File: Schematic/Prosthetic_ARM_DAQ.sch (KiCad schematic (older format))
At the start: 12 parts, among them J1 USB4085-GF-A_REVA, J2 Conn_01x05, U1 STM32F411CEUx

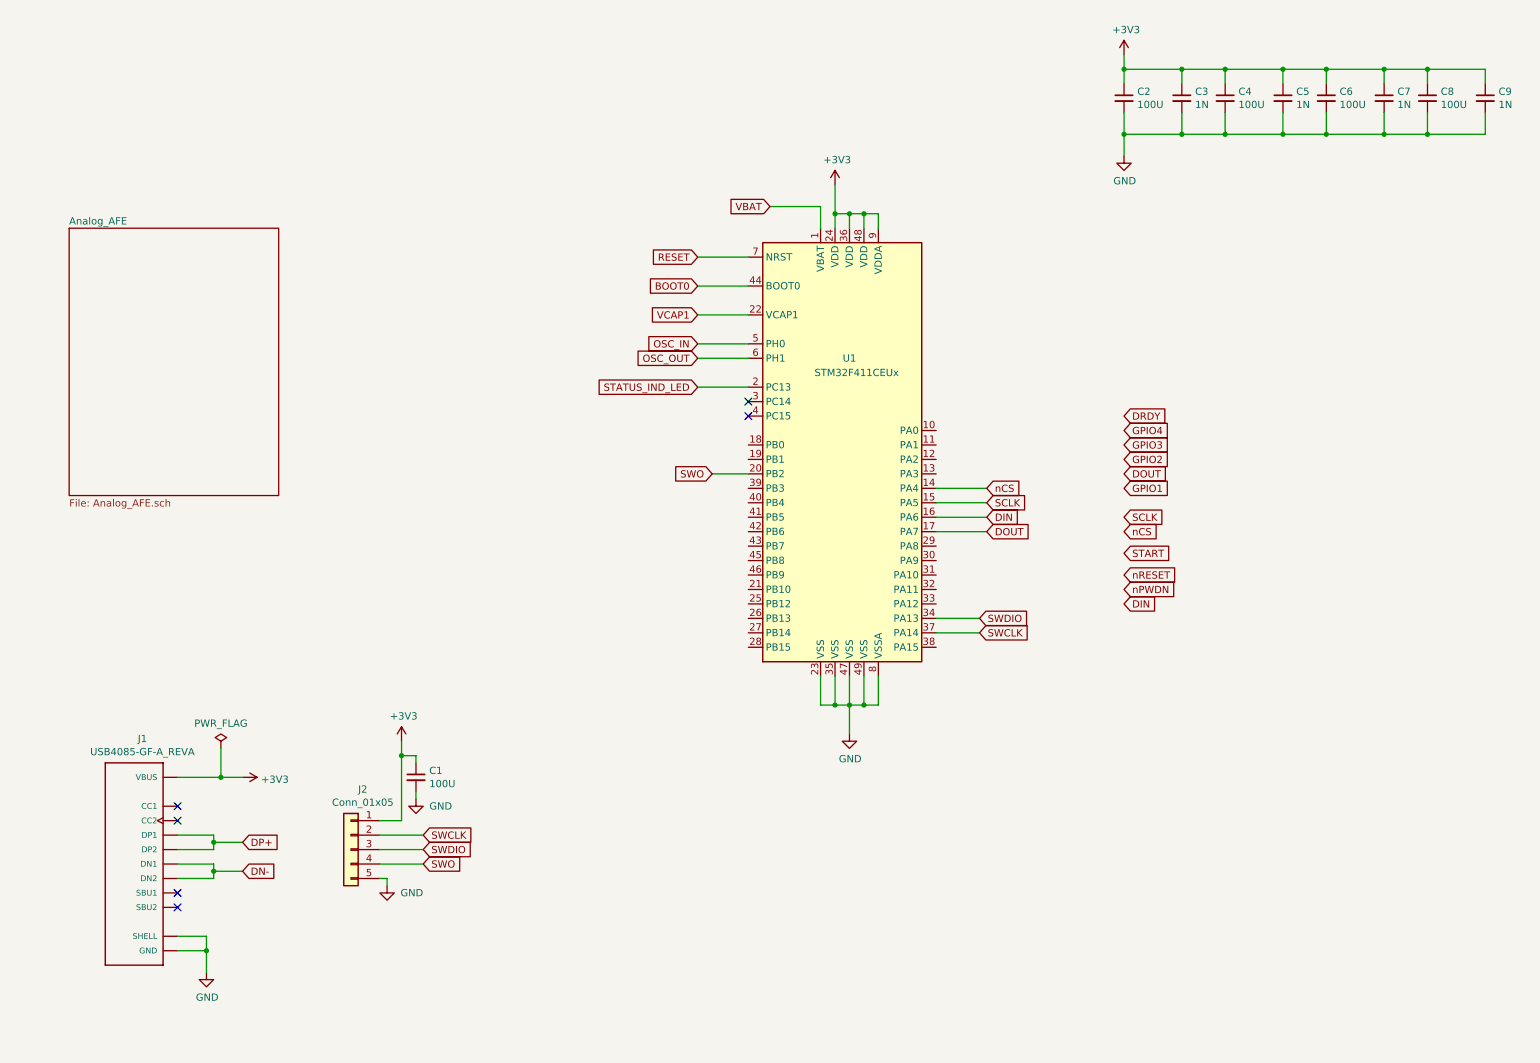
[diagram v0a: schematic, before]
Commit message: Add files via upload
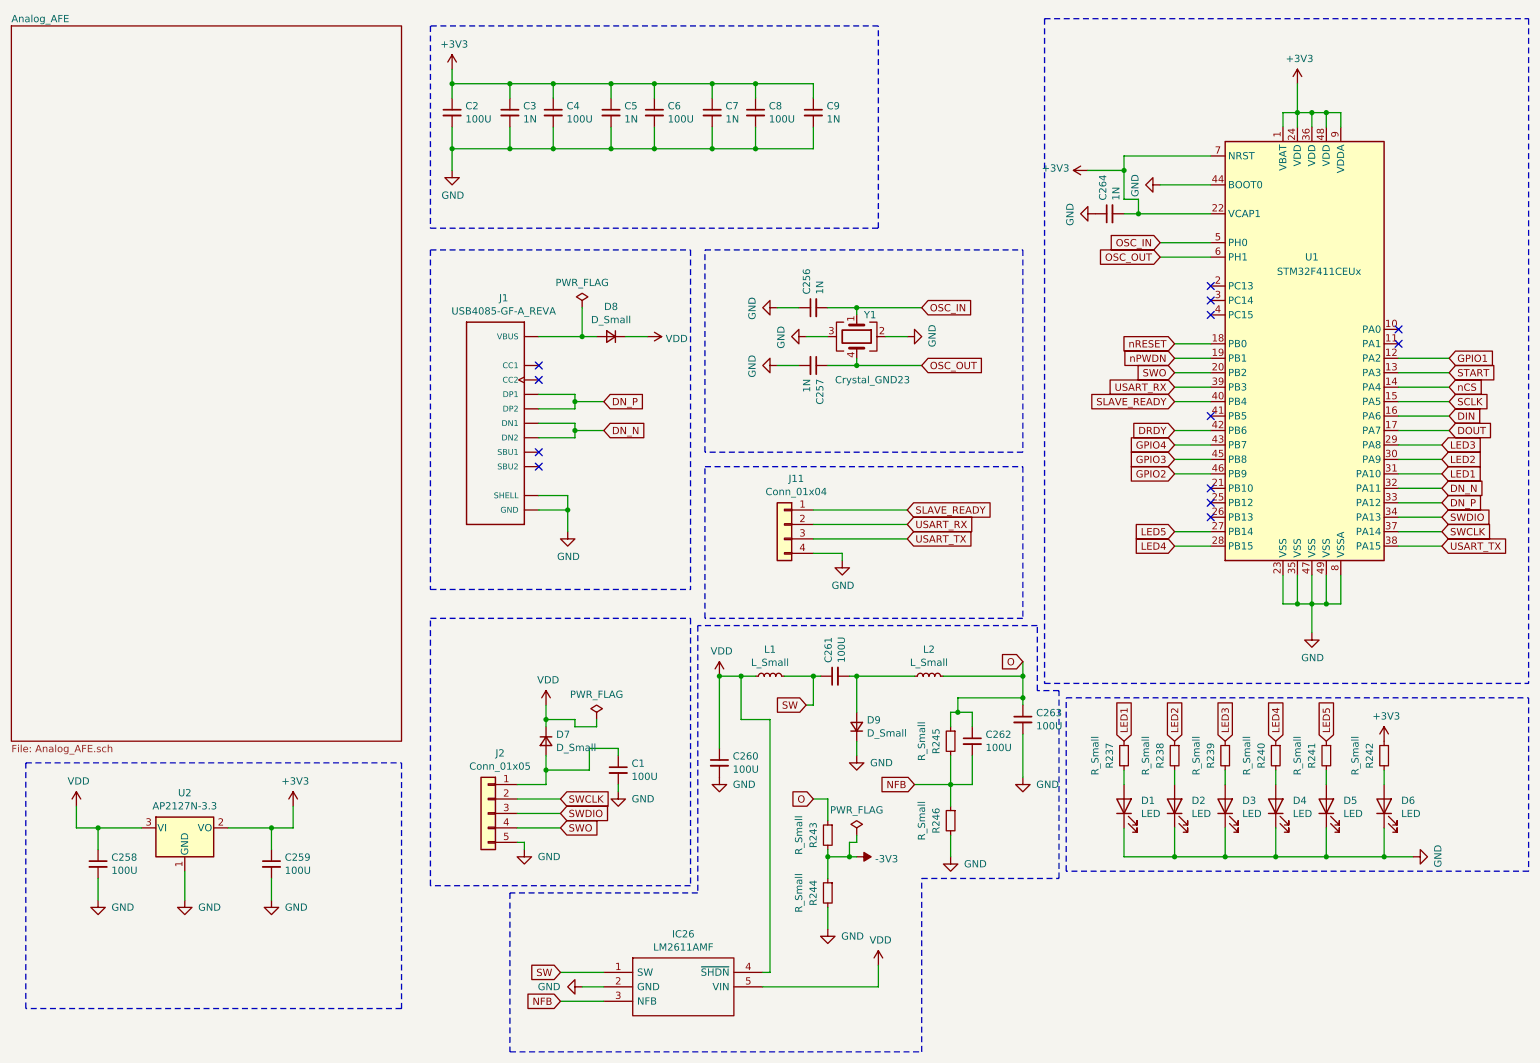
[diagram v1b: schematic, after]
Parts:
- added C256, C257, C264: 1N, Capacitor_SMD:C_0402_1005Metric, symbol Device:C_Small
- added C258, C259, C260, C261, C262, C263: 100U, Capacitor_SMD:C_0402_1005Metric, symbol Device:C_Small
- added D1, D2, D3, D4, D5, D6: LED, LED_SMD:LED_0805_2012Metric_Pad1.15x1.40mm_HandSolder, symbol Device:LED
- added D7, D8, D9: D_Small, Diode_SMD:D_0603_1608Metric_Pad1.05x0.95mm_HandSolder, symbol Device:D_Small
- added IC26: LM2611AMF, ASSETS:SOT95P280X145-5N, symbol Regular_Use:LM2611AMF
- added J11: Conn_01x04, Connector_JST:JST_PH_B4B-PH-SM4-TB_1x04-1MP_P2.00mm_Vertical, symbol Connector_Generic:Conn_01x04
- added L1, L2: L_Small, Inductor_SMD:L_0603_1608Metric_Pad1.05x0.95mm_HandSolder, symbol Device:L_Small
- added R237, R238, R239, R240, R241, R242, R243, R244, R245, R246: R_Small, Resistor_SMD:R_0402_1005Metric, symbol Device:R_Small
- added U2: AP2127N-3.3, Package_TO_SOT_SMD:SOT-23, symbol Regulator_Linear:AP2127N-3.3
- added Y1: Crystal_GND23, Crystal:Crystal_SMD_TXC_7M-4Pin_3.2x2.5mm, symbol Device:Crystal_GND23
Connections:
- net BOOT0 is gone; now on net GND: U1.44 (BOOT0)
- net DN- is gone; now on net DN_N: J1.A7 (DN1), J1.B7 (DN2)
- net DP+ is gone; now on net DN_P: J1.A6 (DP1), J1.B6 (DP2)
- net RESET is gone; now on net +3V3: U1.7 (NRST)
- net VBAT is gone; now on net +3V3: U1.1 (VBAT)
- net VCAP1 is gone; now on net +3V3: U1.22 (VCAP1)
- net +3V3: now also C259.1, C264.2, R242.1, U2.2 (VO); no longer C1.1, J1.A4 (VBUS), J1.A9 (VBUS), J1.B4 (VBUS), J1.B9 (VBUS), J2.1 (Pin_1)
- net DRDY: now also U1.42 (PB6)
- net GND: now also C256.1, C257.2, C258.2, C259.2, C260.2, C263.2, C264.1, D1.1 (K), D2.1 (K), D3.1 (K), D4.1 (K), D5.1 (K), D6.1 (K), D9.1 (K), IC26.2 (GND), J11.4 (Pin_4), R244.2, R246.2, U2.1 (GND), Y1.2, Y1.3
- net GPIO1: now also U1.12 (PA2)
- net GPIO2: now also U1.46 (PB9)
- net GPIO3: now also U1.45 (PB8)
- net GPIO4: now also U1.43 (PB7)
- net OSC_IN: now also C256.2, Y1.1
- net OSC_OUT: now also C257.1, Y1.4
- net START: now also U1.13 (PA3)
- net nPWDN: now also U1.19 (PB1)
- net nRESET: now also U1.18 (PB0)
- net LED5: now reaches U1.27 (PB14)
- net LED5: now also R241.1
- net LED4: now reaches U1.28 (PB15)
- net LED4: now also R240.1
- net LED3: now reaches U1.29 (PA8)
- net LED3: now also R239.1
- net LED2: now reaches U1.30 (PA9)
- net LED2: now also R238.1
- net LED1: now reaches U1.31 (PA10)
- net LED1: now also R237.1
- net DN_N: now reaches U1.32 (PA11)
- net DN_P: now reaches U1.33 (PA12)
- net USART_TX: now reaches U1.38 (PA15)
- net USART_TX: now also J11.3 (Pin_3)
- net USART_RX: now reaches U1.39 (PB3)
- net USART_RX: now also J11.2 (Pin_2)
- net SLAVE_READY: now reaches U1.40 (PB4)
- net SLAVE_READY: now also J11.1 (Pin_1)
- net STATUS_IND_LED: no longer names the net of U1.2 (PC13)
- new net: C1.1, D7.2 (A), J2.1 (Pin_1)
- new net: D8.2 (A), J1.A4 (VBUS), J1.A9 (VBUS), J1.B4 (VBUS), J1.B9 (VBUS)
- new net: D1.2 (A), R237.2
- new net: D2.2 (A), R238.2
- new net: D3.2 (A), R239.2
- new net: D4.2 (A), R240.2
- new net: D5.2 (A), R241.2
- new net: D6.2 (A), R242.2
- new net: C261.2, D9.2 (A), L2.1
- new net -3V3: R243.2, R244.1
- new net NFB: C262.2, IC26.3 (NFB), R245.2, R246.1
- new net O: C262.1, C263.1, L2.2, R243.1, R245.1
- new net SW: C261.1, IC26.1 (SW), L1.2
- new net VDD: C258.1, C260.1, D7.1 (K), D8.1 (K), IC26.4 (~SHDN), IC26.5 (VIN), L1.1, U2.3 (VI)
- no-connect marks 6 -> 13
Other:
- moved on the sheet: C1, C2, C3, C4, C5, C6, C7, C8, C9, J1, J2, U1
